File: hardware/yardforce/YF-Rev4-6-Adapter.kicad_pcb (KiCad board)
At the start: 2 copper layers, 62.3 x 70 mm, 58 parts, among them J1 USB_OTG, J2 TC2050-IDC, J3 YF-Rev6-B, J4 YF-Rev6-A, J5 YF-Rev4-A, J6 YF-Rev4-B, J7 OM UI Board, J8 Shell Stop, J9 Rain, U1 AMS1117-3.3, U3 TCA9555PWR, U4 ESP32-S3-FH4R2, Y1 40MHz 10.5pF ±10ppm

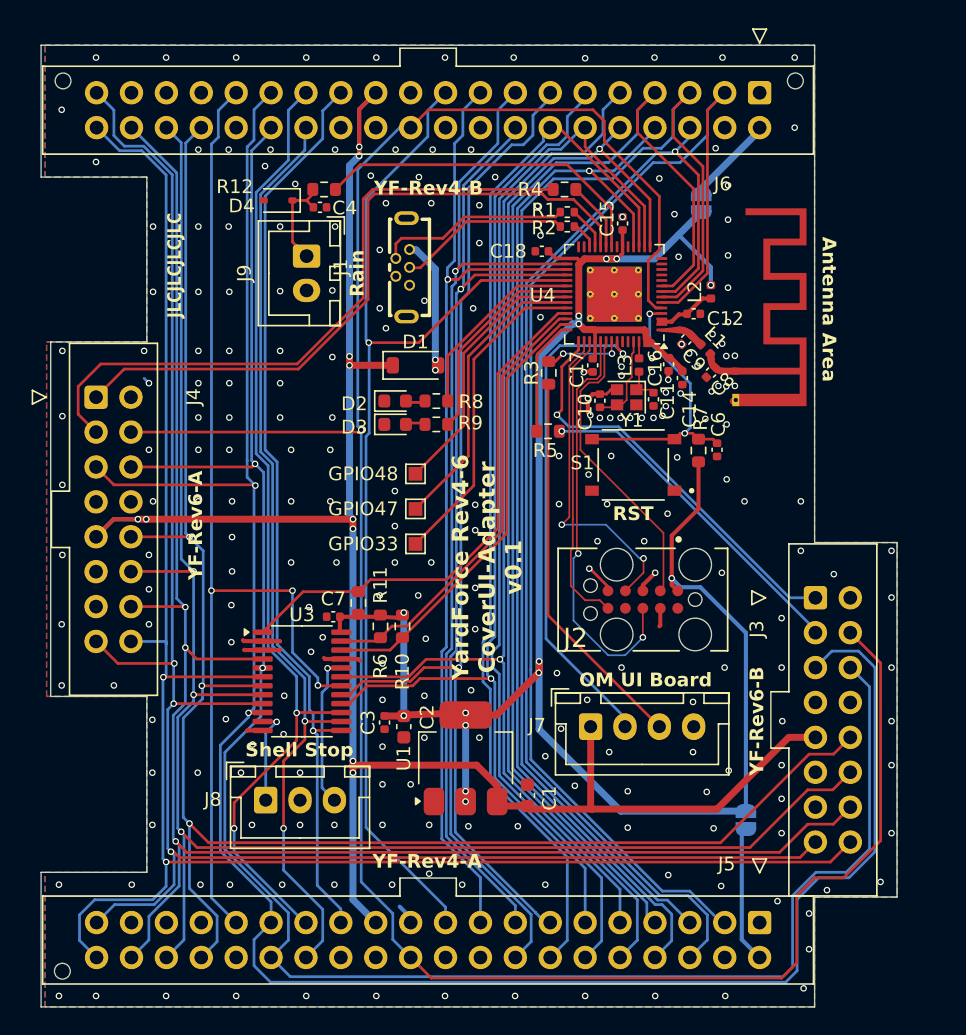
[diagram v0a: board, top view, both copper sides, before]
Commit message: Rev 0.2 hardware
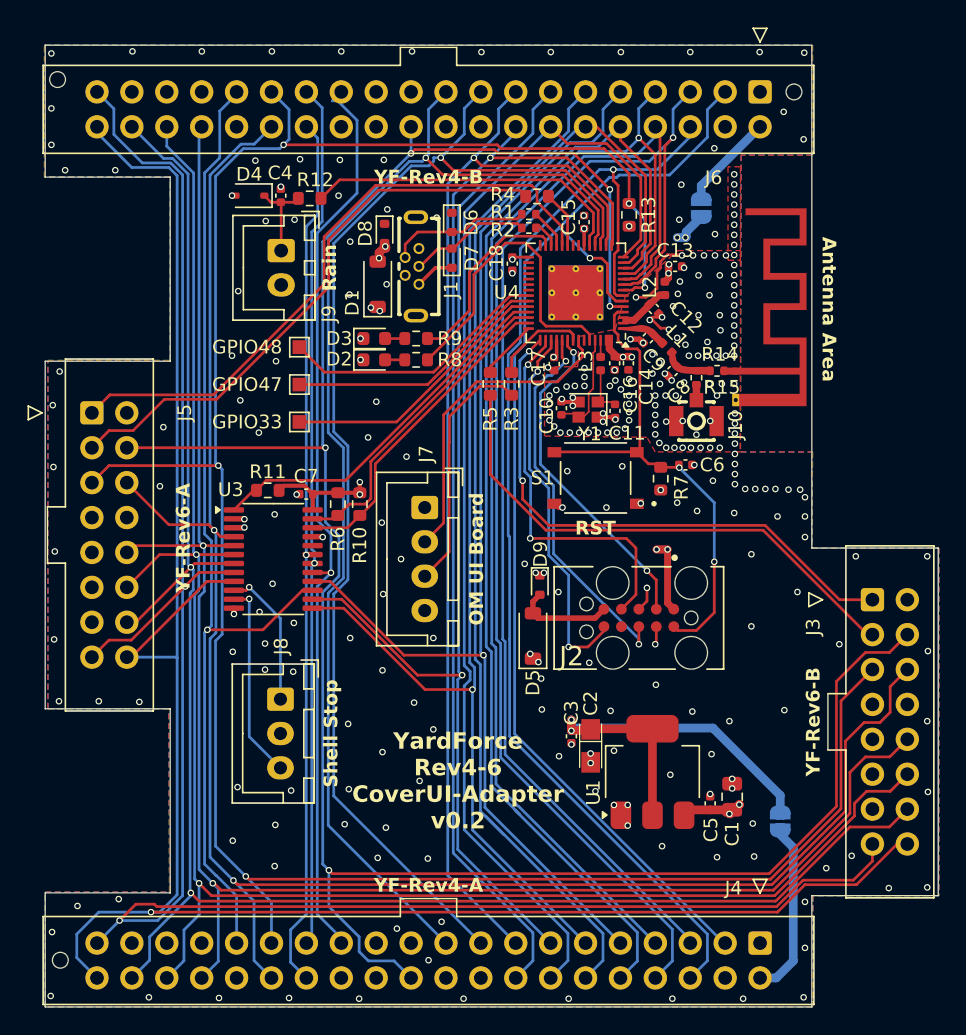
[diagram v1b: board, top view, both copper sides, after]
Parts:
- removed JP3: Rev4-B 3.3V, Jumper:SolderJumper-2_P1.3mm_Open_RoundedPad1.0x1.5mm
- added C13: .1uF, Capacitor_SMD:C_0402_1005Metric, F.Cu at (165.8, 66.1)
- added C5: .1uF, Capacitor_SMD:C_0402_1005Metric, F.Cu at (168.4, 105.2)
- added D5: D_Schottky, Diode_SMD:D_SOD-123, F.Cu at (155.5, 93.0)
- added D6: D_TVS, Diode_SMD:D_SOD-523, F.Cu at (149.6, 62.9)
- added D7: D_TVS, Diode_SMD:D_SOD-523, F.Cu at (149.6, 65.5)
- added D8: D_TVS, Diode_SMD:D_SOD-523, F.Cu at (144.7, 63.7)
- added D9: D_TVS, Diode_SMD:D_SOD-523, F.Cu at (156.0, 89.3)
- added J10: IPEX/U.FL, libs:IPEX-SMD_BWIPX-1-001E, F.Cu at (167.4, 76.6)
- added JP1: Rev4-A 3.3V, Jumper:SolderJumper-2_P1.3mm_Open_RoundedPad1.0x1.5mm, B.Cu at (173.5, 106.5)
- added R13: 10k, Resistor_SMD:R_0603_1608Metric, F.Cu at (162.5, 62.4)
- added R14: 0, Resistor_SMD:R_0402_1005Metric, F.Cu at (168.9, 73.7)
- added R15: 0, Resistor_SMD:R_0402_1005Metric, F.Cu at (167.4, 74.2)
- C1: value 10uF -> 22uF; footprint Capacitor_SMD:C_0603_1608Metric -> Capacitor_SMD:C_0805_2012Metric
- C2: value 10uF -> 22uF/10V; footprint Capacitor_SMD:C_0603_1608Metric -> libs:CASE-A_3216
- J4: value YF-Rev6-A -> YF-Rev4-A; footprint libs:IDC-Hybrid_2x08_P2.54mm_Latch_Vertical -> libs:IDC-Hybrid_2x20_P2.54mm_Latch_Vertical
- J5: value YF-Rev4-A -> YF-Rev6-A; footprint libs:IDC-Hybrid_2x20_P2.54mm_Latch_Vertical -> libs:IDC-Hybrid_2x08_P2.54mm_Latch_Vertical
- JP2: value Rev4-A 3.3V -> Rev4-B 3.3V
- R3, R4, R5: value 22 -> 470
- R8: value 200 -> 220
- moved J4 62.5 mm to (172.0, 115.4), turned to 180 degrees
- moved J5 61.1 mm to (123.5, 76.7), turned to -90 degrees
- moved JP2 44.7 mm to (167.8, 61.9), turned to -90 degrees
- moved J7 20.0 mm to (147.6, 83.7), turned to -90 degrees
- moved C1 14.9 mm to (170.0, 104.7)
- moved C2 13.7 mm to (159.7, 101.0)
- moved C3 13.6 mm to (158.3, 100.3)
- moved U1 13.6 mm to (164.2, 102.9)
- moved GPIO48 12.5 mm to (138.5, 72.0)
- moved GPIO47 12.4 mm to (138.5, 74.7)
- moved GPIO33 12.3 mm to (138.5, 77.4)
- moved R11 10.5 mm to (136.2, 82.4), turned to 0 degrees
- moved R10 9.42 mm to (142.9, 83.4)
- moved R6 9.42 mm to (141.3, 83.4)
- moved U3 9.14 mm to (136.6, 87.4)
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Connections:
- net /JTAG_TCK-SWCLK renamed /JTAG_TCK
- net /JTAG_TDO-SWD renamed /JTAG_TDO
- net /JTAG_TMS-SWDIO renamed /JTAG_TMS
- C6 pad 1: Net-(U4-CHIP_PU/RESET) -> /RESET
- C8 pad 1: Net-(ANT1-Pad1) -> Net-(C8-Pad1)
- J2 pad 10: unconnected-(J2-Pad10) -> /RESET
- J2 pad 5: GND -> Net-(D5-A)
- J4 pad 1: /RXD1 -> GND
- J4 pad 10: /HALL_LIFTX -> /LED_14HR
- J4 pad 11: unconnected-(J4-Pin_11-Pad11) -> /BTN_14HR
- J4 pad 12: /HALL_LBUMP -> /LED_24HR
- J4 pad 13: GND -> /BTN_24HR
- J4 pad 14: /STOP_1 -> /LED_34HR
- J4 pad 15: /HALL_RBUMP -> /LED_S1
- J4 pad 16: /HALL_LIFT -> /LED_LOCK
- J4 pad 2: unconnected-(J4-Pin_2-Pad2) -> Net-(J4-Pin_2)
- J4 pad 3: /TXD1 -> /LED_LIFTED
- J4 pad 4: /BTN_PLAY -> unconnected-(J4-Pin_4-Pad4)
- J4 pad 5: /BTN_HOME -> /LED_CONN
- J4 pad 6: /STOP_2 -> /LED_BAT
- J4 pad 7: GND -> /LED_CHARGE
- J4 pad 8: GND -> /LED_44HR
- J4 pad 9: +5V -> /BTN_44HR
- J5 pad 1: GND -> /RXD1
- J5 pad 10: /LED_4H/LCD -> /HALL_LIFTX
- J5 pad 11: /BTN_4H/R4 -> unconnected-(J5-Pin_11-Pad11)
- J5 pad 12: /LED_6H/LCD -> /HALL_LBUMP
- J5 pad 13: /BTN_6H/R5 -> GND
- J5 pad 14: /LED_8H/R1 -> /STOP_1
- J5 pad 15: /LED_S1/ADS7843_BUSY -> /HALL_RBUMP
- J5 pad 16: /LED_LOCK -> /HALL_LIFT
- J5 pad 2: Net-(J5-Pin_2) -> unconnected-(J5-Pin_2-Pad2)
- J5 pad 3: /LED_LIFTED_ADS7843_CS -> /TXD1
- J5 pad 4: unconnected-(J5-Pin_4-Pad4) -> /BTN_PLAY
- J5 pad 5: /LED_CONN_ADS7843-DIN -> /BTN_HOME
- J5 pad 6: /LED_BAT_ADS7843-DOUT -> /STOP_2
- J5 pad 7: /LED_CHARGE -> GND
- J5 pad 8: /LED_10H/LCD -> GND
- J5 pad 9: /BTN_10H/R3 -> +5V
- J6 pad 10: /LED_4H/LCD -> /LED_14HR
- J6 pad 11: /BTN_4H/R4 -> /BTN_14HR
- J6 pad 12: /LED_6H/LCD -> /LED_24HR
- J6 pad 13: /BTN_6H/R5 -> /BTN_24HR
- J6 pad 14: /LED_8H/R1 -> /LED_34HR
- J6 pad 15: /LED_S1/ADS7843_BUSY -> /LED_S1
- J6 pad 3: /LED_LIFTED_ADS7843_CS -> /LED_LIFTED
- J6 pad 31: /BTN_8H/ADS7843_PEN_IRQ -> /BTN_34HR
- J6 pad 5: /LED_CONN_ADS7843-DIN -> /LED_CONN
- J6 pad 6: /LED_BAT_ADS7843-DOUT -> /LED_BAT
- J6 pad 8: /LED_10H/LCD -> /LED_44HR
- J6 pad 9: /BTN_10H/R3 -> /BTN_44HR
- J8 pad 1: /Shell Stop 1 -> /SHELL_STOP_1
- J8 pad 3: /Shell Stop 2 -> /SHELL_STOP_2
- JP2 pad 1: Net-(J5-Pin_2) -> Net-(J6-Pin_2)
- L1 pad 1: Net-(ANT1-Pad1) -> Net-(C8-Pad1)
- R7 pad 1: Net-(U4-CHIP_PU/RESET) -> /RESET
- S1 pad C: Net-(U4-CHIP_PU/RESET) -> /RESET
- S1 pad D: Net-(U4-CHIP_PU/RESET) -> /RESET
- U3 pad 10: /BTN_HOME -> /SHELL_STOP_1
- U3 pad 11: /Shell Stop 1 -> /SHELL_STOP_2
- U3 pad 13: /BTN_LOCK -> /BTN_14HR
- U3 pad 14: /BTN_S1 -> /BTN_24HR
- U3 pad 15: /BTN_S2 -> /BTN_34HR
- U3 pad 16: /BTN_4H/R4 -> /BTN_44HR
- U3 pad 17: /BTN_6H/R5 -> /BTN_LOCK
- U3 pad 18: /BTN_8H/ADS7843_PEN_IRQ -> /BTN_S2
- U3 pad 19: /BTN_10H/R3 -> /BTN_S1
- U3 pad 20: /Shell Stop 2 -> unconnected-(U3-P17-Pad20)
- U3 pad 4: /STOP_1 -> /STOP_2
- U3 pad 5: /STOP_2 -> /HALL_LIFTX
- U3 pad 6: /HALL_LIFT -> /HALL_LBUMP
- U3 pad 7: /HALL_LIFTX -> /STOP_1
- U3 pad 8: /HALL_LBUMP -> /HALL_RBUMP
- U3 pad 9: /HALL_RBUMP -> /HALL_LIFT
- U4 pad 10: unconnected-(U4-GPIO5/ADC1_CH4-Pad10) -> /LED_44HR
- U4 pad 11: unconnected-(U4-GPIO6/ADC1_CH5-Pad11) -> /LED_CHARGE
- U4 pad 12: unconnected-(U4-GPIO7/ADC1_CH6-Pad12) -> /LED_14HR
- U4 pad 13: unconnected-(U4-GPIO8/ADC1_CH7-Pad13) -> /LED_24HR
- U4 pad 14: unconnected-(U4-GPIO9/ADC1_CH8-Pad14) -> /LED_34HR
- U4 pad 15: /LED_4H/LCD -> /LED_LOCK
- U4 pad 16: /LED_6H/LCD -> /LED_S1
- U4 pad 17: /LED_8H/R1 -> /LED_S2
- U4 pad 18: /LED_10H/LCD -> /LCD_BACKLIGHT
- U4 pad 19: unconnected-(U4-GPIO14/ADC2_CH3-Pad19) -> /RAIN
- U4 pad 22: /RAIN -> unconnected-(U4-GPIO16/ADC2_CH5/XTAL_32K_N-Pad22)
- U4 pad 27: unconnected-(U4-GPIO21-Pad27) -> /LED_RD
- U4 pad 30: /LED_S1/ADS7843_BUSY -> unconnected-(U4-SPIHD/GPIO27-Pad30)
- U4 pad 31: /LED_S2 -> unconnected-(U4-SPIWP/GPIO28-Pad31)
- U4 pad 32: /LED_LOCK -> unconnected-(U4-SPICS0/GPIO29-Pad32)
- U4 pad 33: /LCD_BACKLIGHT -> unconnected-(U4-SPICLK/GPIO30-Pad33)
- U4 pad 34: /LED_GN -> unconnected-(U4-SPIQ/GPIO31-Pad34)
- U4 pad 35: /LED_RD -> unconnected-(U4-SPID/GPIO32-Pad35)
- U4 pad 4: Net-(U4-CHIP_PU/RESET) -> /RESET
- U4 pad 52: unconnected-(U4-GPIO46-Pad52) -> /LED_GN
- U4 pad 6: /LED_LIFTED_ADS7843_CS -> /LED_LIFTED
- U4 pad 7: /LED_CONN_ADS7843-DIN -> /LED_BAT
- U4 pad 8: /LED_BAT_ADS7843-DOUT -> /BTN_HOME
- U4 pad 9: /LED_CHARGE -> /LED_CONN
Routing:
- net /LED_CONN_ADS7843-DIN: track 92.4 -> 0.00 mm
- net /LED_LIFTED_ADS7843_CS: track 92.2 -> 0.00 mm
- net /LED_CONN: track 0.00 -> 88.3 mm, vias 0 -> 1
- net /LED_44HR: track 0.00 -> 86.5 mm
- net /BTN_44HR: track 0.00 -> 86.0 mm, vias 0 -> 1
- net /LED_BAT: track 0.00 -> 85.7 mm, vias 0 -> 1
- net /LED_LIFTED: track 0.00 -> 85.2 mm, vias 0 -> 1
- net /LED_BAT_ADS7843-DOUT: track 85.1 -> 0.00 mm, vias 1 -> 0
- net /LED_14HR: track 0.00 -> 84.8 mm
- net /LED_24HR: track 0.00 -> 84.5 mm
- net /BTN_14HR: track 0.00 -> 83.2 mm, vias 0 -> 1
- net /LED_34HR: track 0.00 -> 82.9 mm
- net /BTN_24HR: track 0.00 -> 81.0 mm, vias 0 -> 1
- net /BTN_10H/R3: track 80.5 -> 0.00 mm, vias 1 -> 0
- net /LED_S1: track 0.00 -> 80.2 mm, vias 0 -> 1
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- added copper zone on In1.Cu, net GND
- added copper zone on In2.Cu, net GND
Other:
- board size 62.3 x 70 mm -> 65 x 70 mm
- copper layers 2 -> 4
- board text added: "YardForce Rev4-6 CoverUI-Adapter v0.2"
- board text removed: "YardForce Rev4-6 CoverUI-Adapter v0.1"
